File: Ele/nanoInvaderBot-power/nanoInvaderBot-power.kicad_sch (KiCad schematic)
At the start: 22 parts, among them J1 S6B-ZR-SM4A-TF(LF)(SN), J2 S6B-ZR-SM4A-TF(LF)(SN), J3 1746142-1, J4 Conn_01x20, P1 USB_C_Plug_USB2.0, U4 BQ25170DSGR, U5 TLV61048DBVT

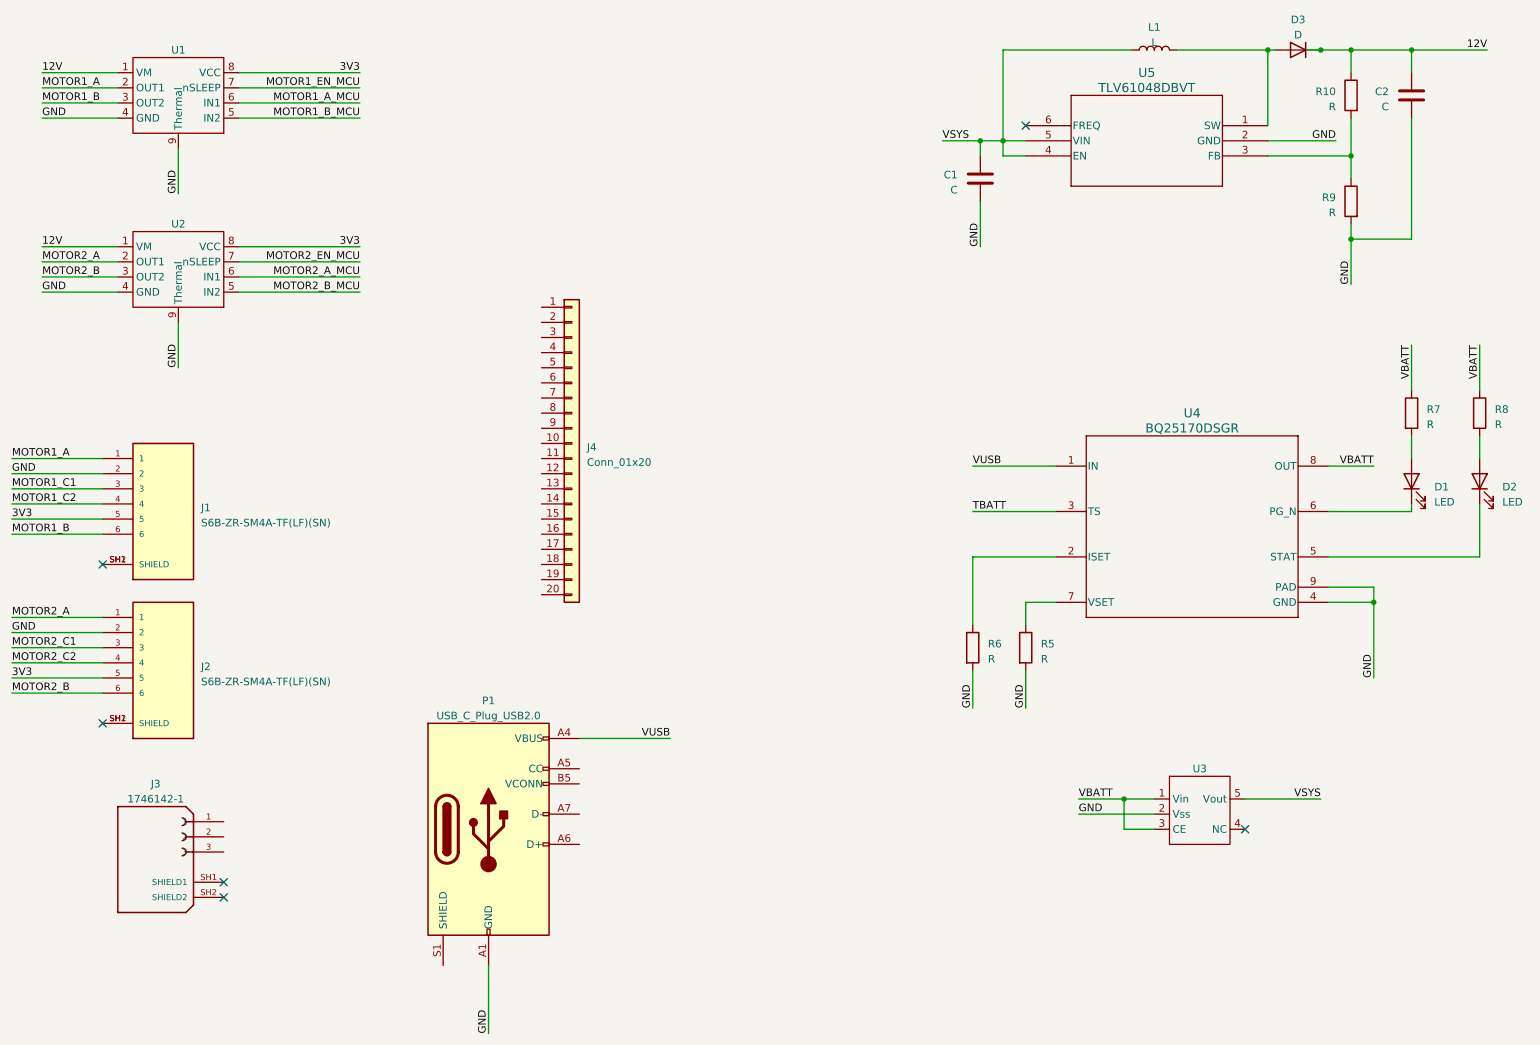
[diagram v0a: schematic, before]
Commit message: Intermediate state -power layer almost done
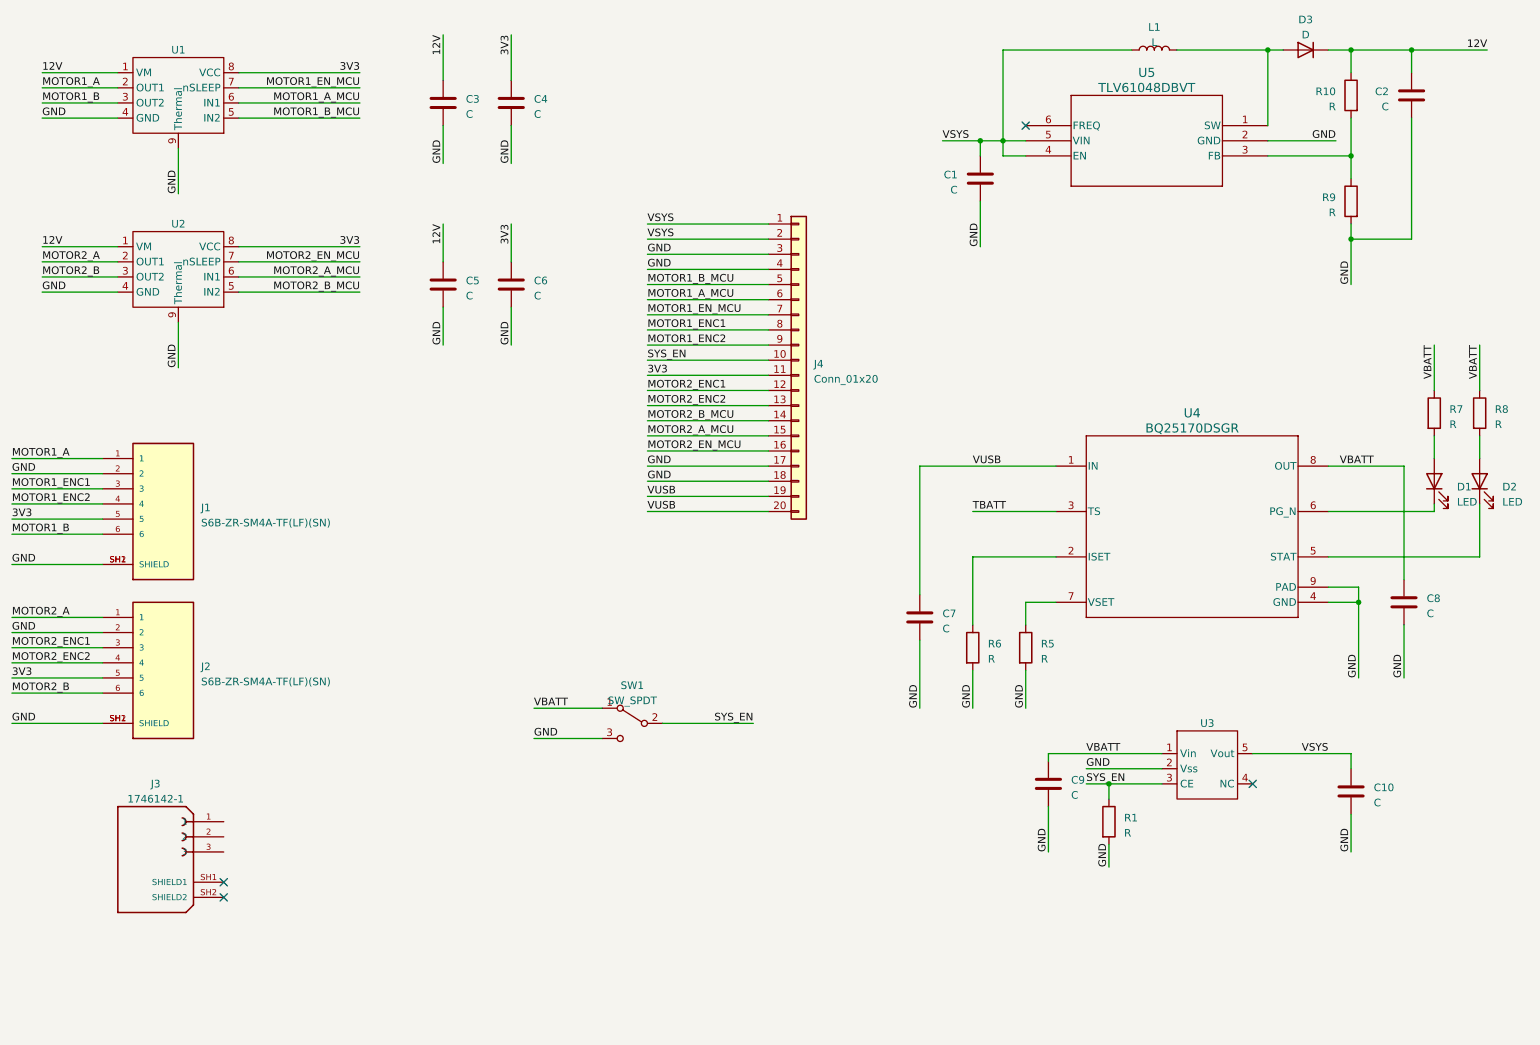
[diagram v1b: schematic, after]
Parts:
- removed P1: USB_C_Plug_USB2.0, Connector_USB:USB_C_Receptacle_GCT_USB4135-GF-A_6P_TopMnt_Horizontal, symbol Connector:USB_C_Plug_USB2.0
- added C10, C4, C6, C7, C8, C9: C, Capacitor_SMD:C_0603_1608Metric, symbol Device:C
- added C3, C5: C, Capacitor_SMD:C_1210_3225Metric, symbol Device:C
- added R1: R, Resistor_SMD:R_0402_1005Metric, symbol Device:R
- added SW1: SW_SPDT, Button_Switch_SMD:SW_SPDT_PCM12, symbol Switch:SW_SPDT
- C1: footprint (none) -> Capacitor_SMD:C_1210_3225Metric; MPN (none) -> GCM32ER71E106KA57L
- C2: footprint (none) -> Capacitor_SMD:C_1210_3225Metric
- D1, D2: footprint LED_SMD:LED_0603_1608Metric -> Resistor_SMD:R_0402_1005Metric
- D3: footprint (none) -> footprints:SDO_B120AF_DIO
- L1: footprint (none) -> footprints:IND_SWPA5040S_SNL
- R10, R9: footprint (none) -> Resistor_SMD:R_0402_1005Metric
- R5, R6, R7, R8: footprint Resistor_SMD:R_0603_1608Metric -> Resistor_SMD:R_0402_1005Metric
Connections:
- net MOTOR1_C1 is gone; now on net MOTOR1_ENC1: J1.3
- net MOTOR1_C2 is gone; now on net MOTOR1_ENC2: J1.4
- net MOTOR2_C1 is gone; now on net MOTOR2_ENC1: J2.3
- net MOTOR2_C2 is gone; now on net MOTOR2_ENC2: J2.4
- net 12V: now also C3.1, C5.1
- net 3V3: now also J4.11 (Pin_11), C4.1, C6.1
- net GND: now also J1.SH1 (SHIELD), J1.SH2 (SHIELD), J2.SH1 (SHIELD), J2.SH2 (SHIELD), J4.17 (Pin_17), J4.18 (Pin_18), J4.3 (Pin_3), J4.4 (Pin_4), C10.2, C3.2, C4.2, C5.2, C6.2, C7.2, C8.2, C9.2, R1.2, SW1.3 (C)
- net MOTOR1_A_MCU: now also J4.6 (Pin_6)
- net MOTOR1_B_MCU: now also J4.5 (Pin_5)
- net MOTOR1_EN_MCU: now also J4.7 (Pin_7)
- net MOTOR2_A_MCU: now also J4.15 (Pin_15)
- net MOTOR2_B_MCU: now also J4.14 (Pin_14)
- net MOTOR2_EN_MCU: now also J4.16 (Pin_16)
- net VBATT: now also C8.1, C9.1, SW1.1 (A); no longer U3.3 (CE)
- net VSYS: now also J4.1 (Pin_1), J4.2 (Pin_2), C10.1
- net VUSB: now also J4.19 (Pin_19), J4.20 (Pin_20), C7.1
- net SYS_EN: now reaches J4.10 (Pin_10)
- net SYS_EN: now also U3.3 (CE), R1.1, SW1.2 (B)
- net MOTOR2_ENC1: now reaches J4.12 (Pin_12)
- net MOTOR2_ENC2: now reaches J4.13 (Pin_13)
- net MOTOR1_ENC1: now reaches J4.8 (Pin_8)
- net MOTOR1_ENC2: now reaches J4.9 (Pin_9)
- no-connect marks 6 -> 4
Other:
- moved on the sheet: D1, D3, J4, R7, U3
